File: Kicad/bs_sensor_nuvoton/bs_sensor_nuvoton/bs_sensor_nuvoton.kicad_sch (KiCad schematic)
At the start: 20 parts, among them J1 Conn_01x02, J2 Conn_01x04, J3 Conn_01x04, J4 Conn_01x04, U1 NRF24L01_Breakout, U2 AMS1117-3.3, U3 STM32F030F4Px, U4 N76E003AT20, Y1 16MHz

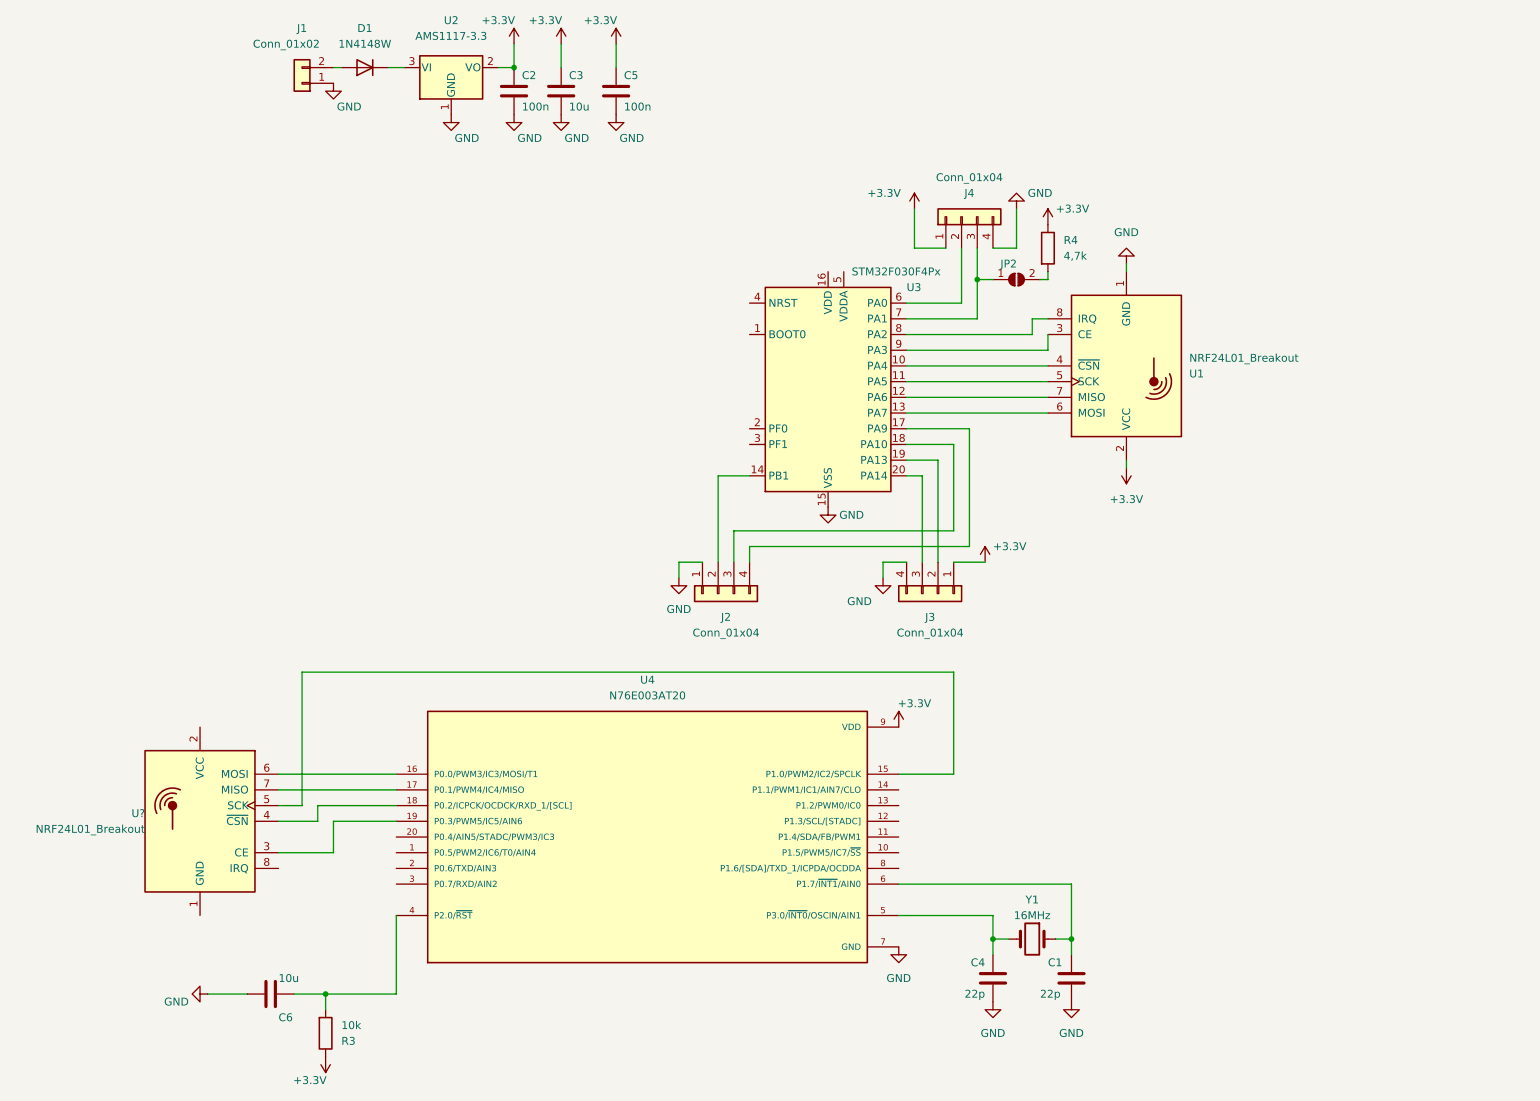
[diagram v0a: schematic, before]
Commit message: 07.09.2022
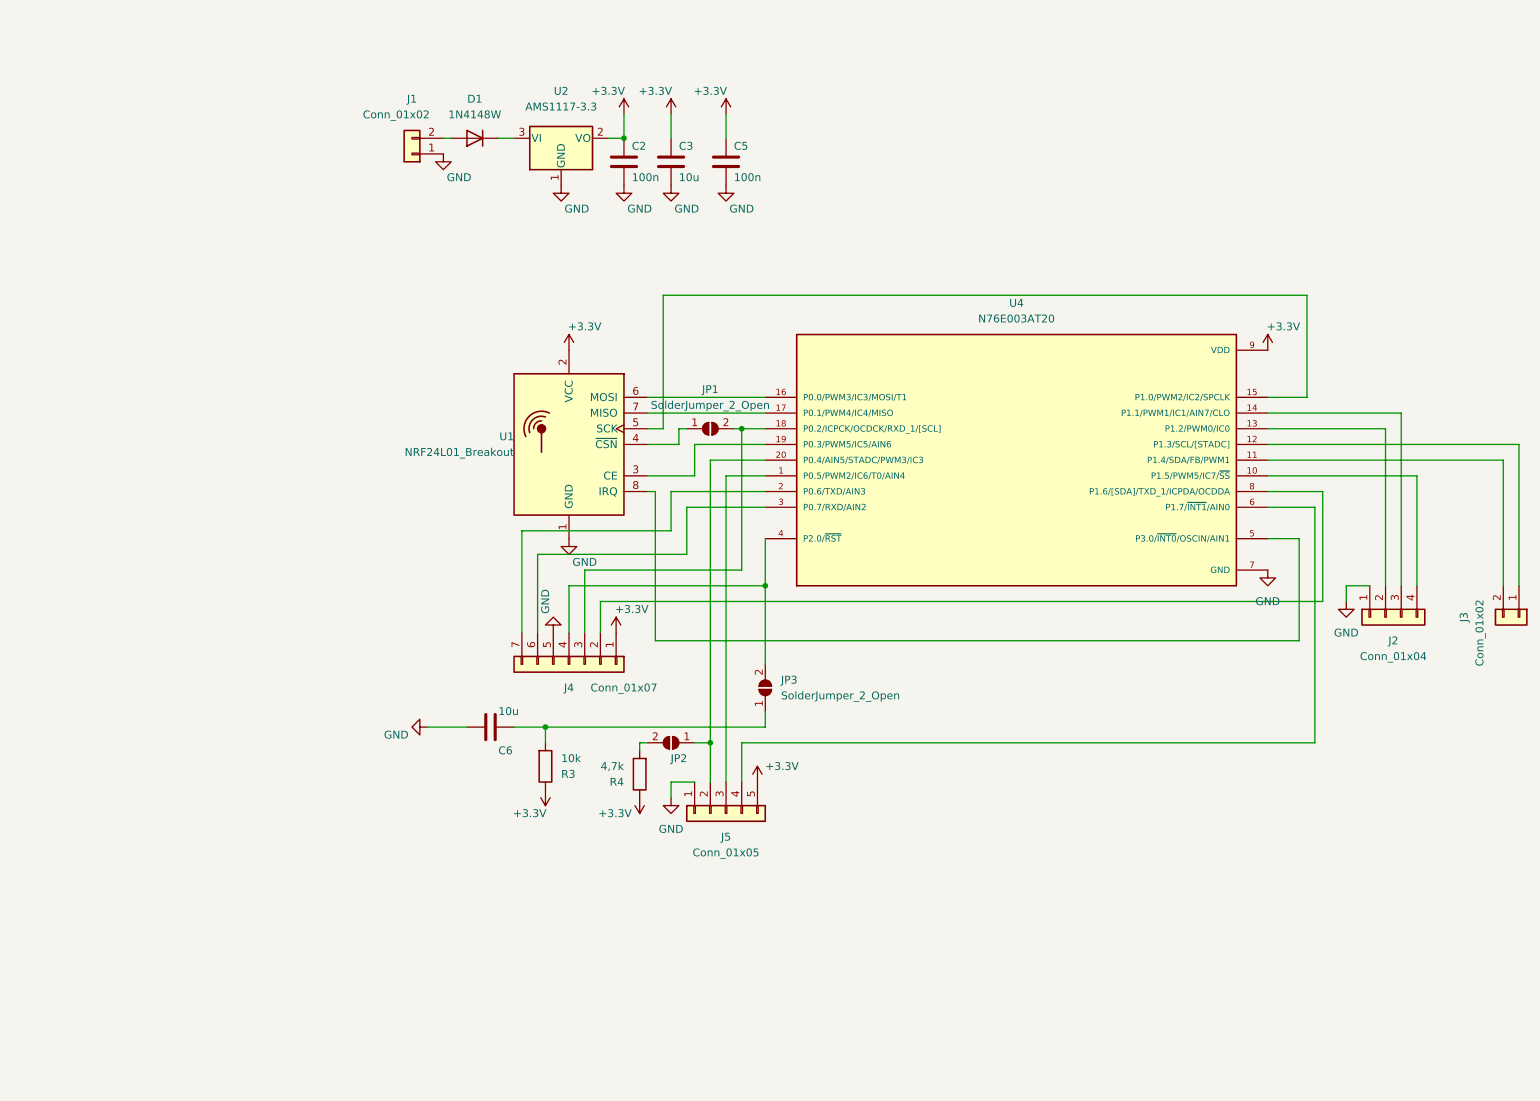
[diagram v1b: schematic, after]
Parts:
- removed C1, C4: 22p, Capacitor_SMD:C_0805_2012Metric, symbol Device:C
- removed J3, J4: Conn_01x04, Connector_PinHeader_2.54mm:PinHeader_1x04_P2.54mm_Vertical, symbol Connector_Generic:Conn_01x04
- removed U1: NRF24L01_Breakout, RF_Module:nRF24L01_Breakout, symbol RF:NRF24L01_Breakout
- removed U3: STM32F030F4Px, Package_SO:TSSOP-20_4.4x6.5mm_P0.65mm, symbol MCU_ST_STM32F0:STM32F030F4Px
- removed Y1: 16MHz, Crystal:Crystal_HC49-U_Vertical, symbol Device:Crystal
- added J3: Conn_01x02, Connector_PinHeader_2.54mm:PinHeader_1x02_P2.54mm_Vertical, symbol Connector_Generic:Conn_01x02
- added J4: Conn_01x07, Connector_PinHeader_2.54mm:PinHeader_1x07_P2.54mm_Vertical, symbol Connector_Generic:Conn_01x07
- added J5: Conn_01x05, Connector_PinHeader_2.54mm:PinHeader_1x05_P2.54mm_Vertical, symbol Connector_Generic:Conn_01x05
- added JP1, JP3: SolderJumper_2_Open, Jumper:SolderJumper-2_P1.3mm_Open_TrianglePad1.0x1.5mm, symbol Jumper:SolderJumper_2_Open
- gave numbers to parts that had none: 1
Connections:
- net +3V3: now also U1.2 (VCC), J4.1 (Pin_1), J5.5 (Pin_5)
- net GND: now also U1.1 (GND), J4.5 (Pin_5), J5.1 (Pin_1)
- net at JP2.1 (A): now also U4.20 (P0.4/AIN5/STADC/PWM3/IC3), J5.2 (Pin_2)
- net at J2.2 (Pin_2): now also U4.13 (P1.2/PWM0/IC0)
- net at J2.4 (Pin_4): now also U4.10 (P1.5/PWM5/IC7/~{SS})
- net at J2.3 (Pin_3): now also U4.14 (P1.1/PWM1/IC1/AIN7/CLO)
- net at U4.18 (P0.2/ICPCK/OCDCK/RXD_1/[SCL]): now also J4.3 (Pin_3), JP1.2 (B); no longer U1.4 (~{CSN})
- net at U1.8 (IRQ): now also U4.5 (P3.0/~{INT0}/OSCIN/AIN1)
- net at C6.1, R3.2: now also JP3.1 (A); no longer U4.4 (P2.0/~{RST})
- net at U4.6 (P1.7/~{INT1}/AIN0): now also J5.4 (Pin_4)
- net at U4.1 (P0.5/PWM2/IC6/T0/AIN4): now also J5.3 (Pin_3)
- net at U4.11 (P1.4/SDA/FB/PWM1): now also J3.2 (Pin_2)
- net at U4.12 (P1.3/SCL/[STADC]): now also J3.1 (Pin_1)
- net at U4.2 (P0.6/TXD/AIN3): now also J4.7 (Pin_7)
- net at U4.3 (P0.7/RXD/AIN2): now also J4.6 (Pin_6)
- net at U4.8 (P1.6/[SDA]/TXD_1/ICPDA/OCDDA): now also J4.2 (Pin_2)
- new net: J4.4 (Pin_4), JP3.2 (B), U4.4 (P2.0/~{RST})
- new net: JP1.1 (A), U1.4 (~{CSN})
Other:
- moved on the sheet: C2, C3, C5, C6, D1, J1, J2, JP2, R3, R4, U1, U2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
